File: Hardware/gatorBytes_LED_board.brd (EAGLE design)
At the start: 110.5 x 57.1 mm, 119 parts

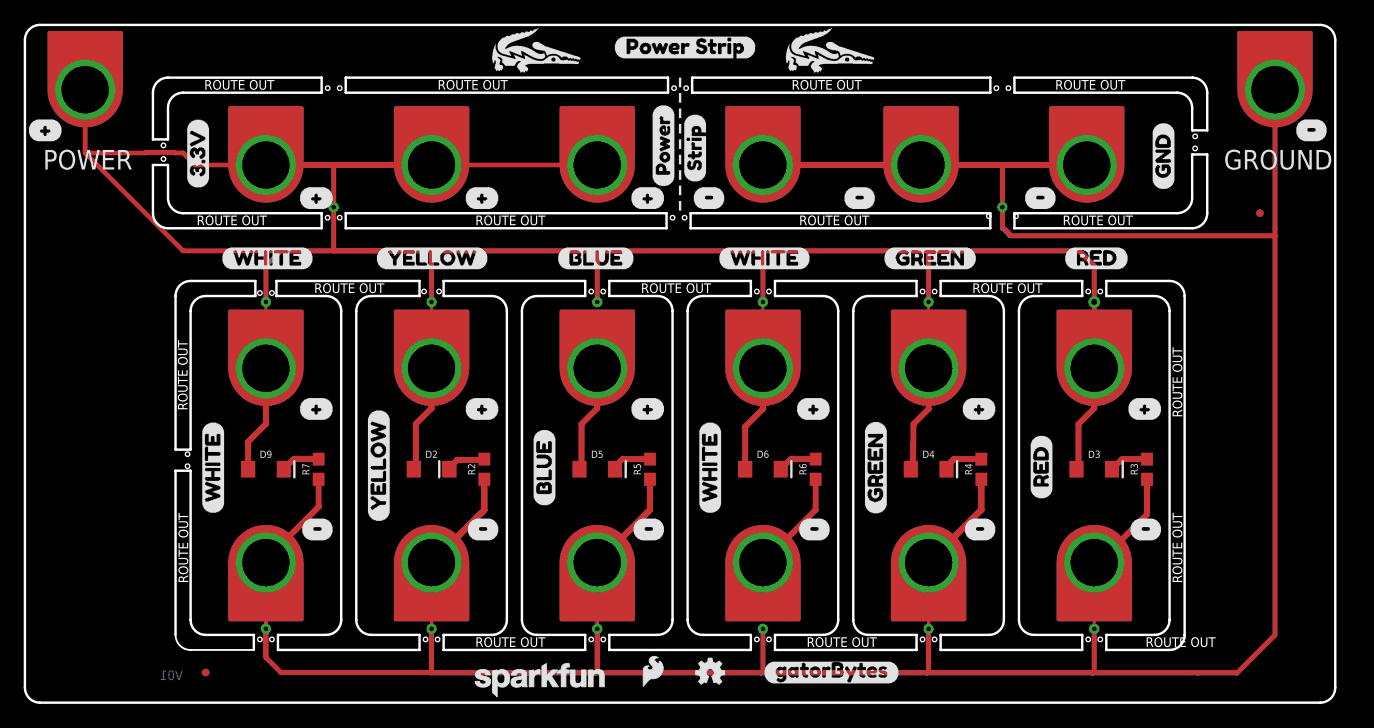
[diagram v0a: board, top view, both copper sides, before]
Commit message: pre design review
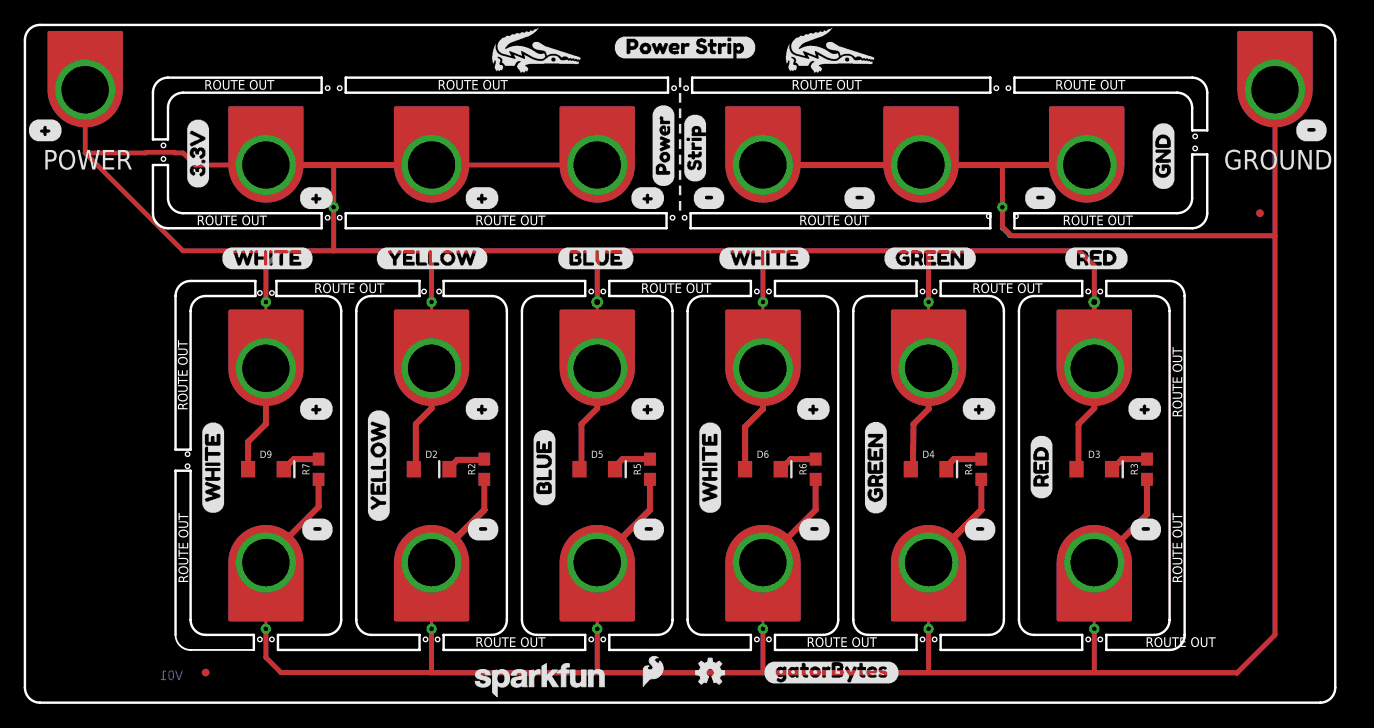
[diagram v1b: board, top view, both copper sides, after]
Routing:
- net GND: track 682.2 -> 632.8 mm
- net 3.3V: track 382.6 -> 374.1 mm, vias 7 -> 8
